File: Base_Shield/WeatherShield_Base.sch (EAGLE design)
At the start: 71 parts, among them Q1 BSS138, Q2 BSS138, U1 DS3231SN, U2 LT3652, U3 TMP100MDBVREP, U4 ADS1015IDGST

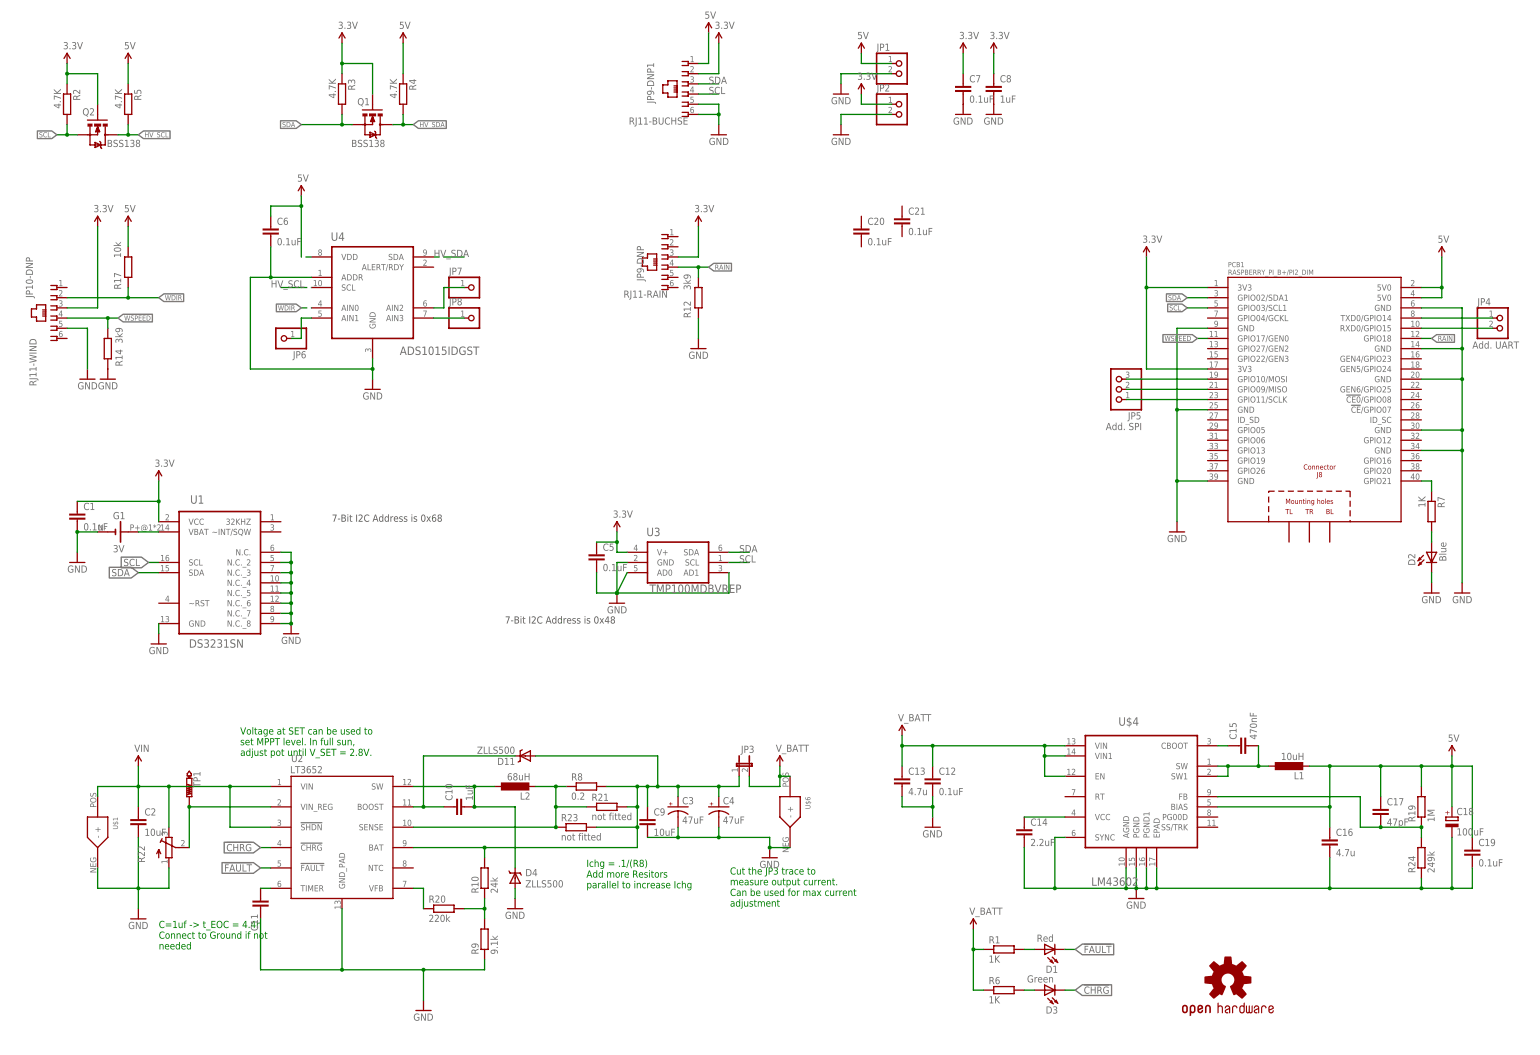
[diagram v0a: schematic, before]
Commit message: WeatherShield_v1
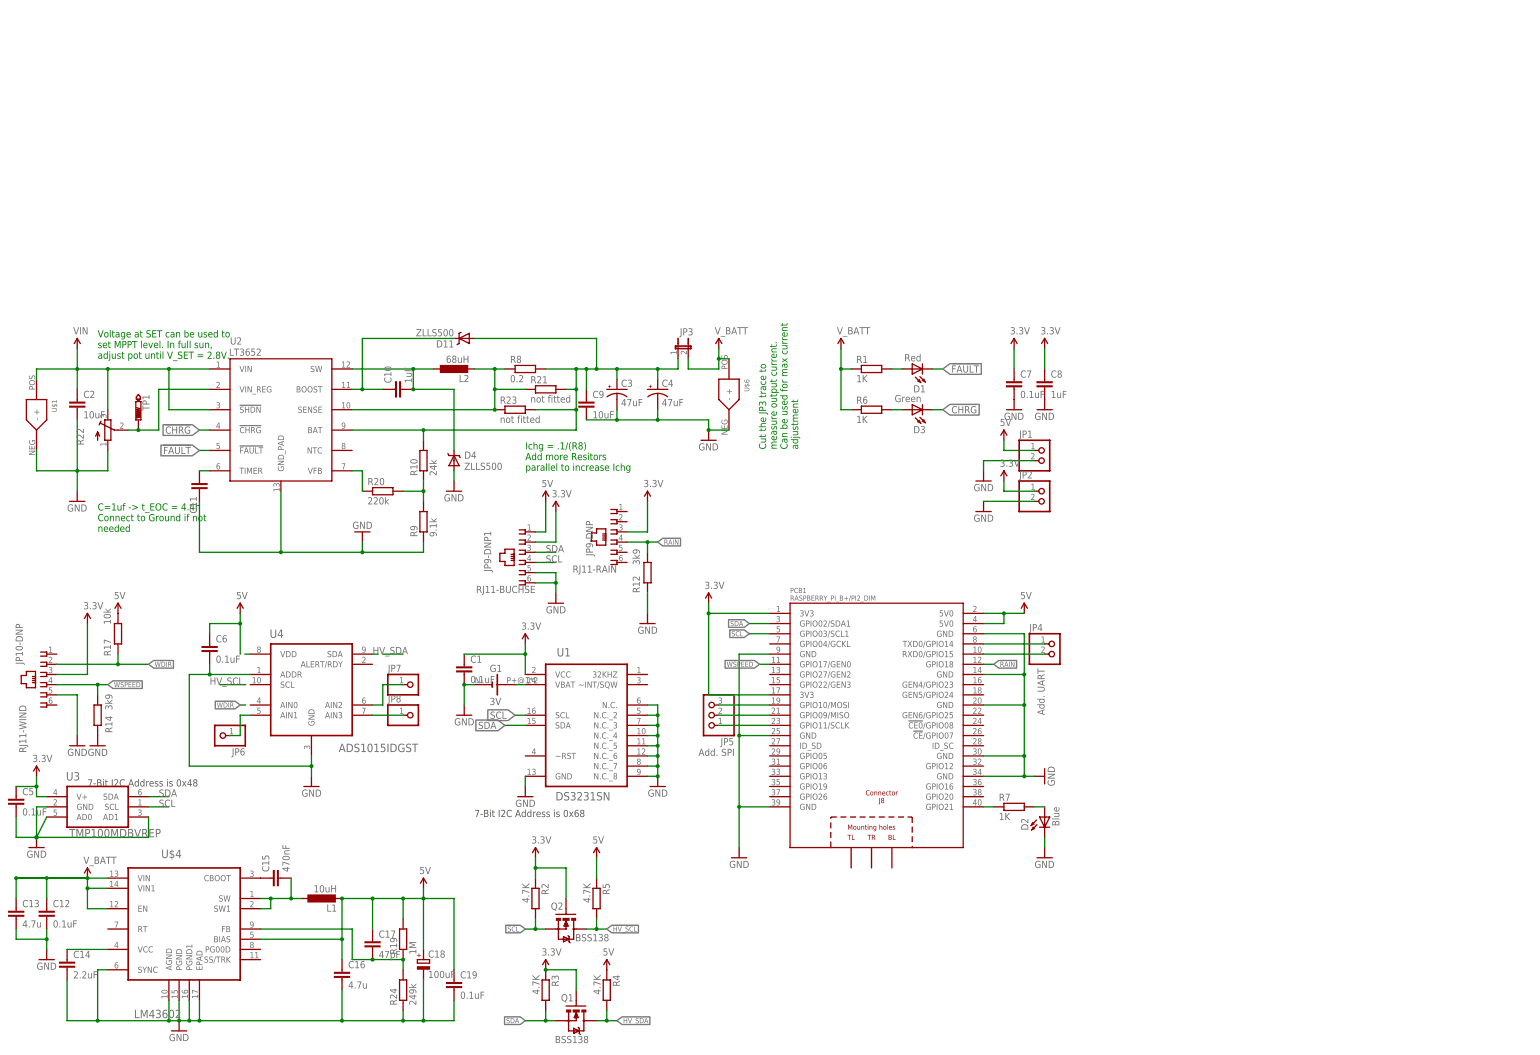
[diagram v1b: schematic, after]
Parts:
- removed C20, C21: 0.1uF, rcl:C-EUC0603
- removed LOGO1: OSHW-LOGOM, SparkFun-Aesthetics:OSHW-LOGOM
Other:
- note added: "+5V Generation (Raspberry Power)"
- moved on the sheet: C1, C10, C11, C12, C13, C14, C15, C16, C17, C18, C19, C2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
